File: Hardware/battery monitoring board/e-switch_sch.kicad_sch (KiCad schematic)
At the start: 5 parts, among them K1 Relay_SPST-NO, Q2 PN2222A

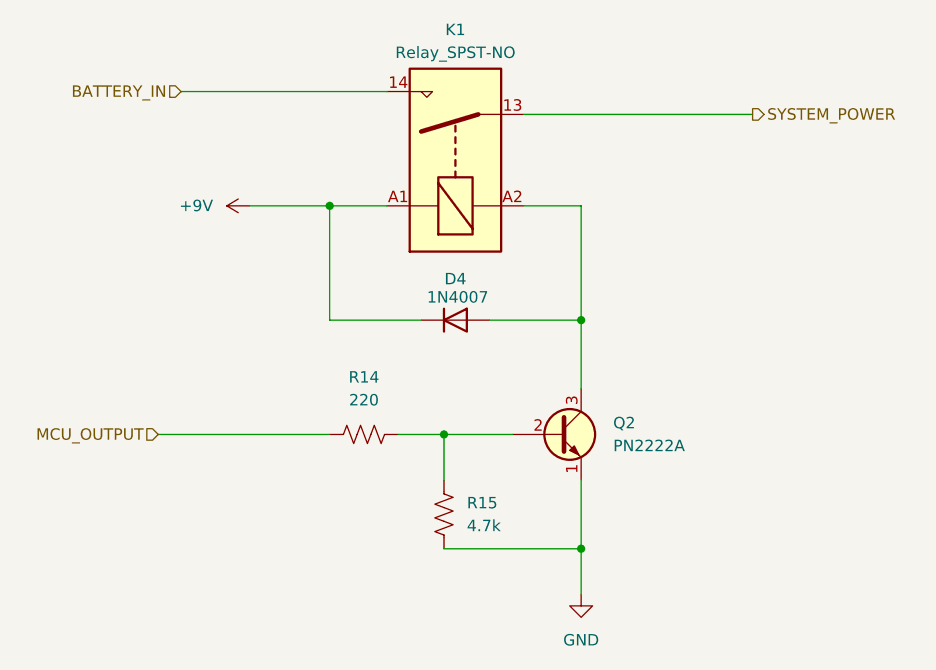
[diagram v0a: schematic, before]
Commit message: Revert "Updated reference labels"
This reverts commit 7ccd23260c988ead49c0bcfa936e50f6d09a7000.
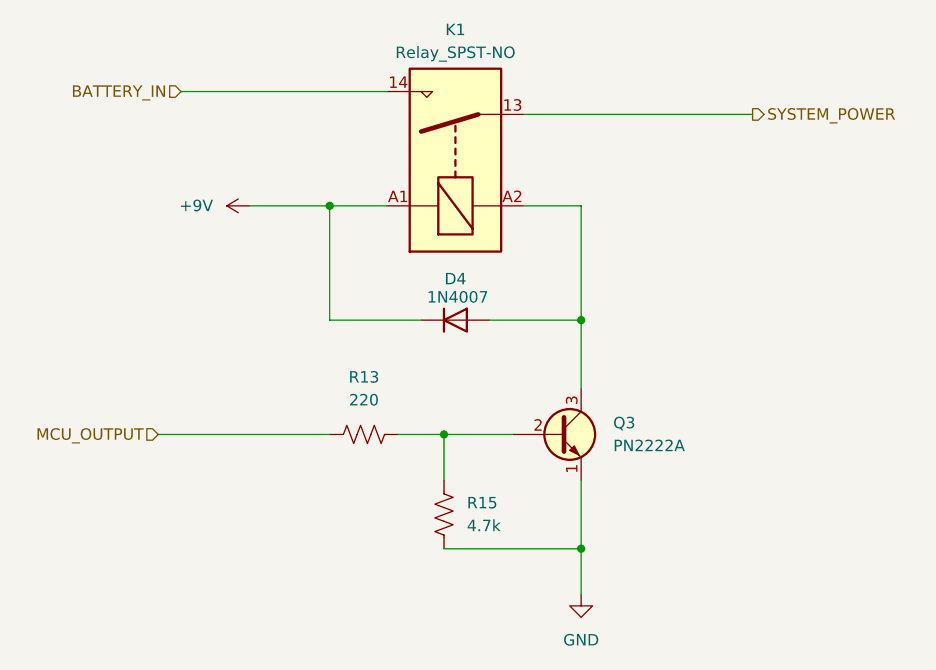
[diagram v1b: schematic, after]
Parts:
- renumbered Q2 to Q3, R14 to R13
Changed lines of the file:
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@@
   (symbol (lib_id "power:GND") (at 86.36 88.9 0) (unit 1)
     (in_bom yes) (on_board yes) (dnp no) (fields_autoplaced)
-    (property "Reference" "#PWR023" (at 86.36 95.25 0)
+    (property "Reference" "#PWR018" (at 86.36 95.25 0)
       (effects (font (size 1.27 1.27)) hide)
     )
@@
       (project "battery monitoring board"
         (path "/bf623d80-ca5a-491f-9daa-4dffbeba5279/d1e89632-1041-42ed-815d-03472eda859a"
-          (reference "#PWR023") (unit 1)
+          (reference "#PWR018") (unit 1)
         )
       )
@@
   (symbol (lib_id "PCM_Transistor_BJT_AKL:PN2222A") (at 83.82 71.12 0) (unit 1)
     (in_bom yes) (on_board yes) (dnp no) (fields_autoplaced)
-    (property "Reference" "Q2" (at 89.916 69.85 0)
+    (property "Reference" "Q3" (at 89.916 69.85 0)
       (effects (font (size 1.27 1.27)) (justify left))
     )
@@
       (project "battery monitoring board"
         (path "/bf623d80-ca5a-491f-9daa-4dffbeba5279/d1e89632-1041-42ed-815d-03472eda859a"
-          (reference "Q2") (unit 1)
+          (reference "Q3") (unit 1)
         )
       )
@@
   (symbol (lib_id "Device:R_US") (at 62.23 71.12 90) (unit 1)
     (in_bom yes) (on_board yes) (dnp no) (fields_autoplaced)
-    (property "Reference" "R14" (at 62.23 64.77 90)
+    (property "Reference" "R13" (at 62.23 64.77 90)
       (effects (font (size 1.27 1.27)))
     )
@@
       (project "battery monitoring board"
         (path "/bf623d80-ca5a-491f-9daa-4dffbeba5279/d1e89632-1041-42ed-815d-03472eda859a"
-          (reference "R14") (unit 1)
+          (reference "R13") (unit 1)
         )
       )
@@
   (symbol (lib_id "PCM_4ms_Power-symbol:+9V") (at 49.53 45.72 90) (unit 1)
     (in_bom yes) (on_board yes) (dnp no) (fields_autoplaced)
-    (property "Reference" "#PWR022" (at 53.34 45.72 0)
+    (property "Reference" "#PWR024" (at 53.34 45.72 0)
       (effects (font (size 1.27 1.27)) hide)
     )
@@
       (project "battery monitoring board"
         (path "/bf623d80-ca5a-491f-9daa-4dffbeba5279/d1e89632-1041-42ed-815d-03472eda859a"
-          (reference "#PWR022") (unit 1)
+          (reference "#PWR024") (unit 1)
         )
       )
